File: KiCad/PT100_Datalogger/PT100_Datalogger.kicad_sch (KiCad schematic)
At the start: 37 parts, among them SW3 SW_Push_Shielded, SW4 SW_Push_Shielded, SW5 SW_Push_Shielded, SW6 SW_Push_Shielded, SW7 SW_Push_Shielded, U1 ESP32-S3-WROOM-1-N8R2, U11 PCF85263AT, U12 FM24CL16B-GTR, U13 MCP9601, Y1 32.768K12.5PI/3215E

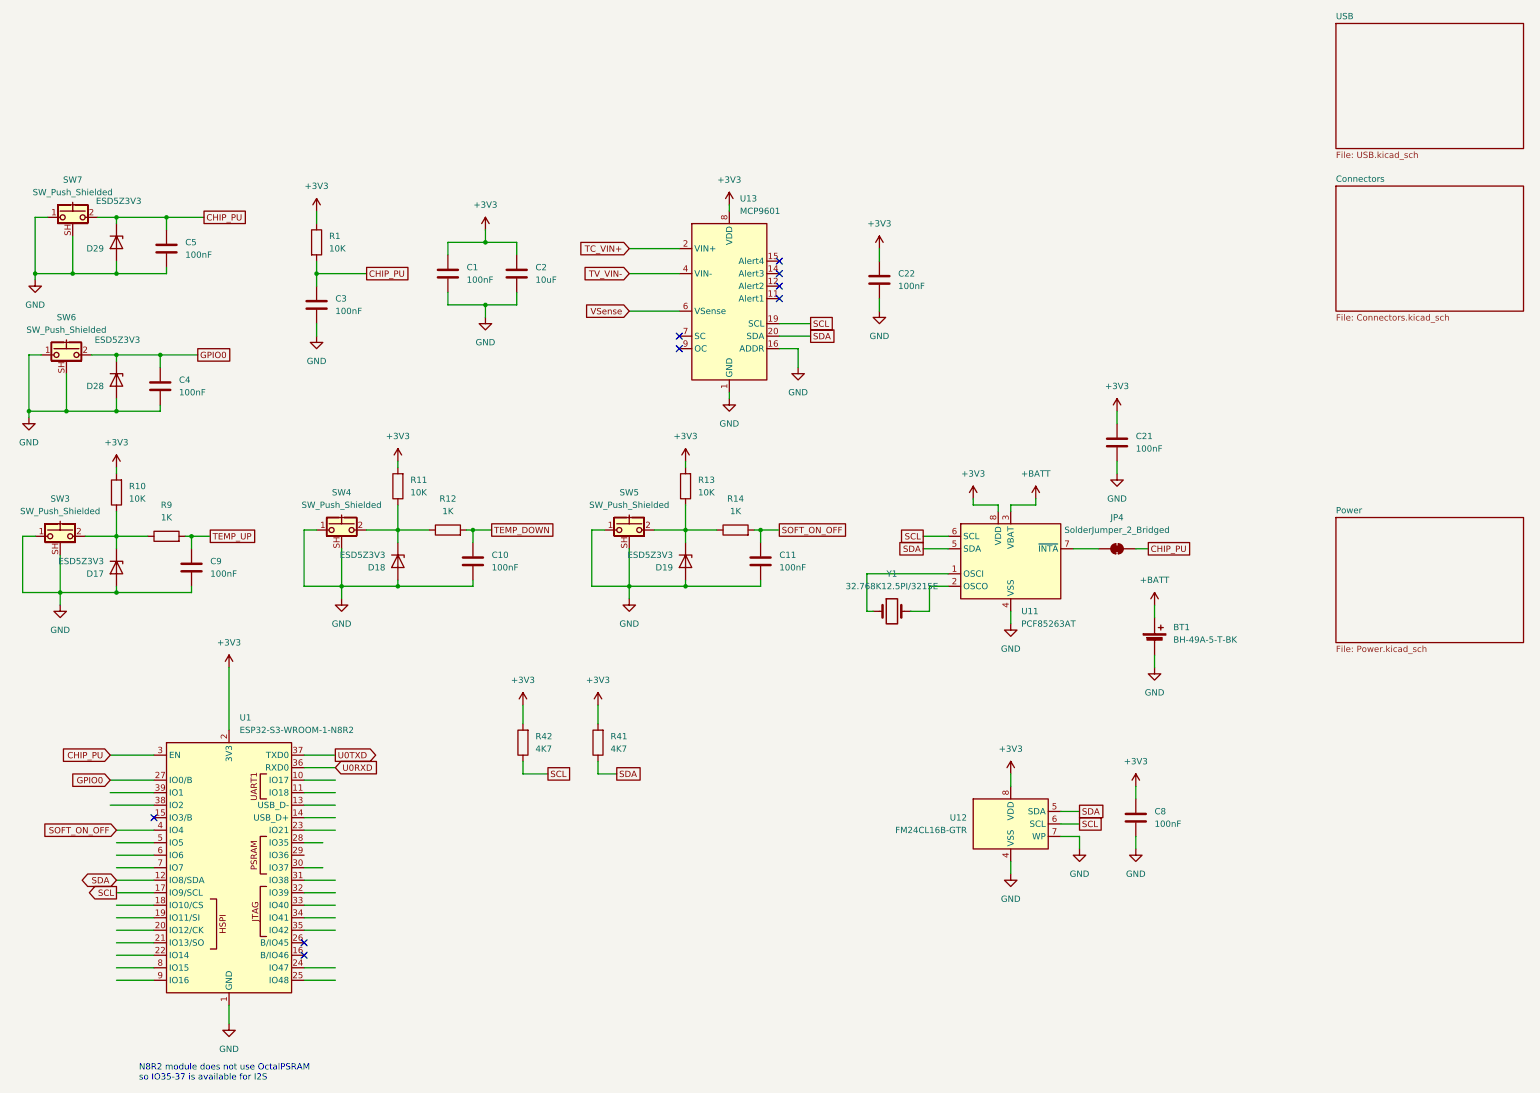
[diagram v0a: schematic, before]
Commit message: Finished KiCad PCB REV A
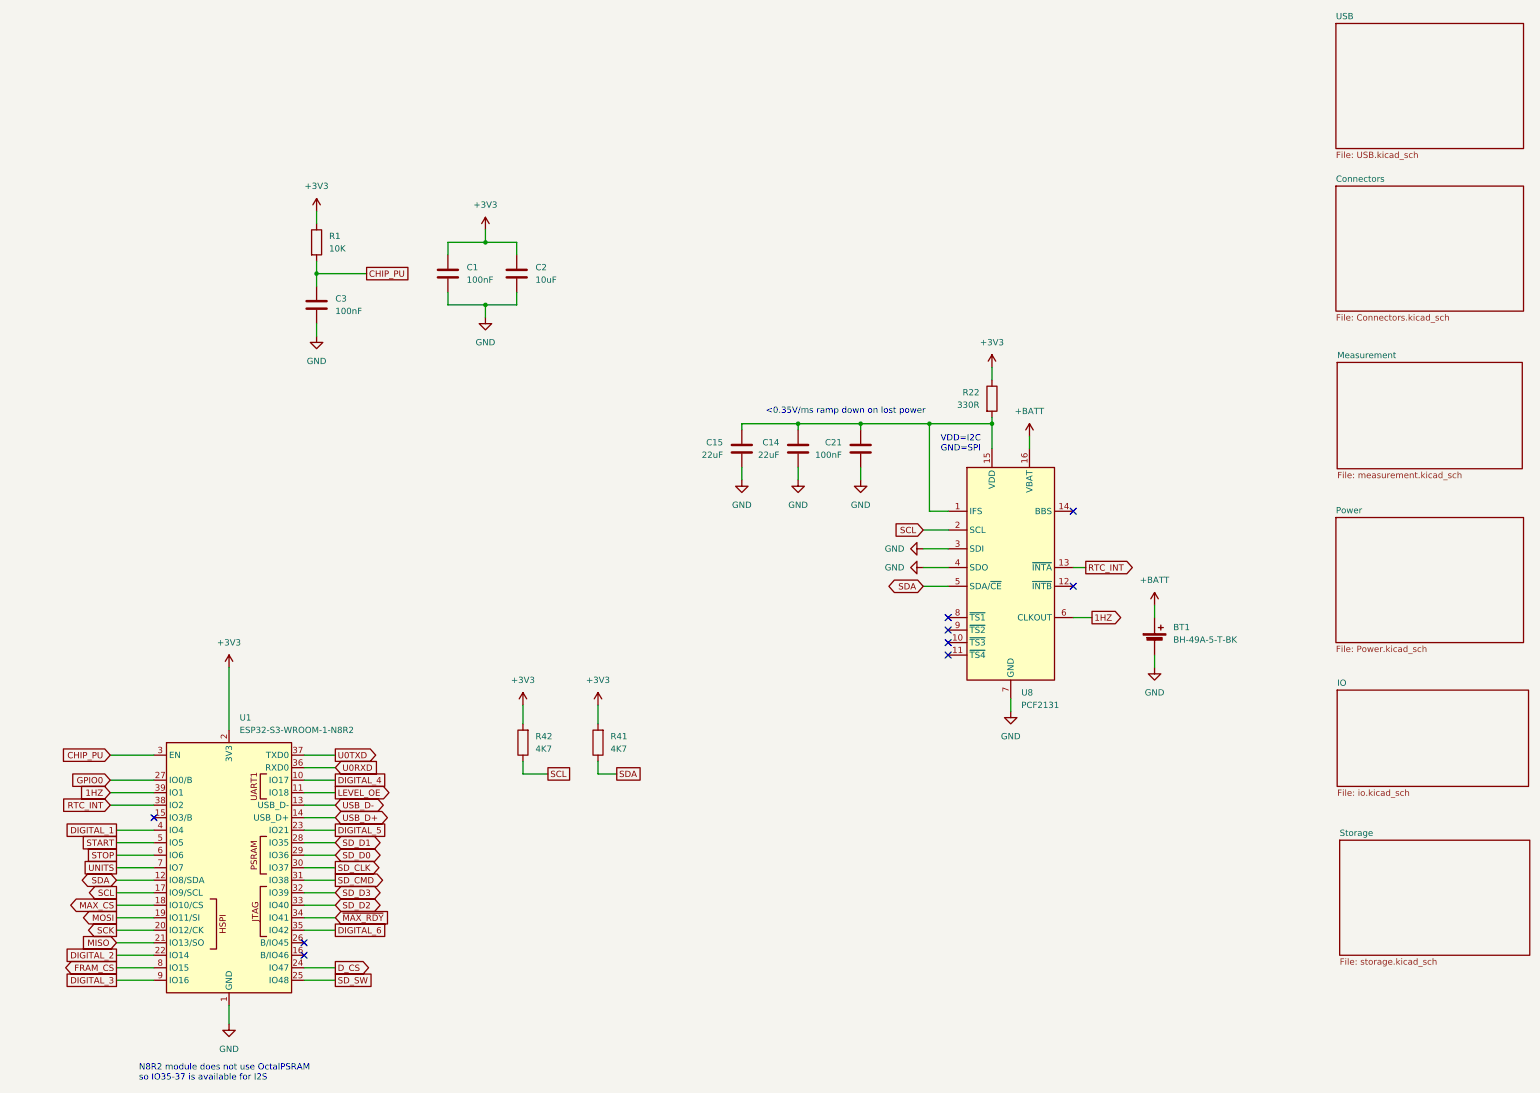
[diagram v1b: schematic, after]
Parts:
- removed C10, C11, C22, C4, C5, C8, C9: 100nF, Capacitor_SMD:C_0603_1608Metric_Pad1.08x0.95mm_HandSolder, symbol Device:C
- removed D17, D18, D19, D28, D29: ESD5Z3V3, Diode_SMD:D_SOD-523, symbol Diode:ESD5Zxx
- removed JP4: SolderJumper_2_Bridged, Jumper:SolderJumper-2_P1.3mm_Bridged_Pad1.0x1.5mm, symbol Jumper:SolderJumper_2_Bridged
- removed R10, R11, R13: 10K, Resistor_SMD:R_0603_1608Metric_Pad0.98x0.95mm_HandSolder, symbol Device:R
- removed R12, R14, R9: 1K, Resistor_SMD:R_0603_1608Metric_Pad0.98x0.95mm_HandSolder, symbol Device:R
- removed SW3, SW4, SW5, SW6, SW7: SW_Push_Shielded, Personal:SW_1825955-6_TEC, symbol Switch:SW_Push_Shielded
- removed U11: PCF85263AT, Package_SO:SOIC-8_3.9x4.9mm_P1.27mm, symbol Timer_RTC:PCF85263AT
- removed U12: FM24CL16B-GTR, Package_SO:SOIC-8_3.9x4.9mm_P1.27mm, symbol Memory_NVRAM:FM24CL16B
- removed U13: MCP9601, Package_DFN_QFN:Texas_RGW0020A_VQFN-20-1EP_5x5mm_P0.65mm_EP3.15x3.15mm_ThermalVias, symbol Personal:MCP9601
- removed Y1: 32.768K12.5PI/3215E, Crystal:Crystal_SMD_3215-2Pin_3.2x1.5mm, symbol Device:Crystal
- added C14, C15: 22uF, Capacitor_SMD:C_0805_2012Metric_Pad1.18x1.45mm_HandSolder, symbol Device:C
- added R22: 330R, Resistor_SMD:R_0603_1608Metric_Pad0.98x0.95mm_HandSolder, symbol Device:R
- added U8: PCF2131, Personal:16-HLSON, symbol Personal:PCF2131
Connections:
- net +3V3: now also R22.1; no longer C21.1
- net +BATT: now also U8.16 (VBAT)
- net SCL: now also U8.2 (SCL)
- net SDA: now also U8.5 (SDA/~{CE})
- net DIGITAL_4: now reaches U1.10 (IO17)
- net LEVEL_OE: now reaches U1.11 (IO18)
- net USB_D-: now reaches U1.13 (USB_D-)
- net USB_D+: now reaches U1.14 (USB_D+)
- net MAX_CS: now reaches U1.18 (IO10/CS)
- net MOSI: now reaches U1.19 (IO11/SI)
- net SCK: now reaches U1.20 (IO12/CK)
- net MISO: now reaches U1.21 (IO13/SO)
- net DIGITAL_2: now reaches U1.22 (IO14)
- net DIGITAL_5: now reaches U1.23 (IO21)
- net D_CS: now reaches U1.24 (IO47)
- net SD_SW: now reaches U1.25 (IO48)
- net SD_D1: now reaches U1.28 (IO35)
- net SD_D0: now reaches U1.29 (IO36)
- net SD_CLK: now reaches U1.30 (IO37)
- net SD_CMD: now reaches U1.31 (IO38)
- net SD_D3: now reaches U1.32 (IO39)
- net SD_D2: now reaches U1.33 (IO40)
- net ~{MAX_RDY}: now reaches U1.34 (IO41)
- net DIGITAL_6: now reaches U1.35 (IO42)
- net RTC_INT: now reaches U1.38 (IO2)
- net RTC_INT: now also U8.13 (~{INTA})
- net 1HZ: now reaches U1.39 (IO1)
- net 1HZ: now also U8.6 (CLKOUT)
- net START: now reaches U1.5 (IO5)
- net STOP: now reaches U1.6 (IO6)
- net UNITS: now reaches U1.7 (IO7)
- net FRAM_CS: now reaches U1.8 (IO15)
- net DIGITAL_3: now reaches U1.9 (IO16)
- net EP renamed GND
- net GND: now also C14.2, C15.2, U8.3 (SDI), U8.4 (SDO), U8.7 (GND)
- net SOFT_ON_OFF renamed DIGITAL_1
- new net: C14.1, C15.1, C21.1, R22.2, U8.1 (IFS), U8.15 (VDD)
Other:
- added sheet IO (io.kicad_sch)
- added sheet Measurement (measurement.kicad_sch)
- added sheet Storage (storage.kicad_sch)
- note added: "<0.35V/ms ramp down on lost power"
- note added: "VDD=I2C GND=SPI"
- moved on the sheet: C21
